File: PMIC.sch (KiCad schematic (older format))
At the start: 63 parts

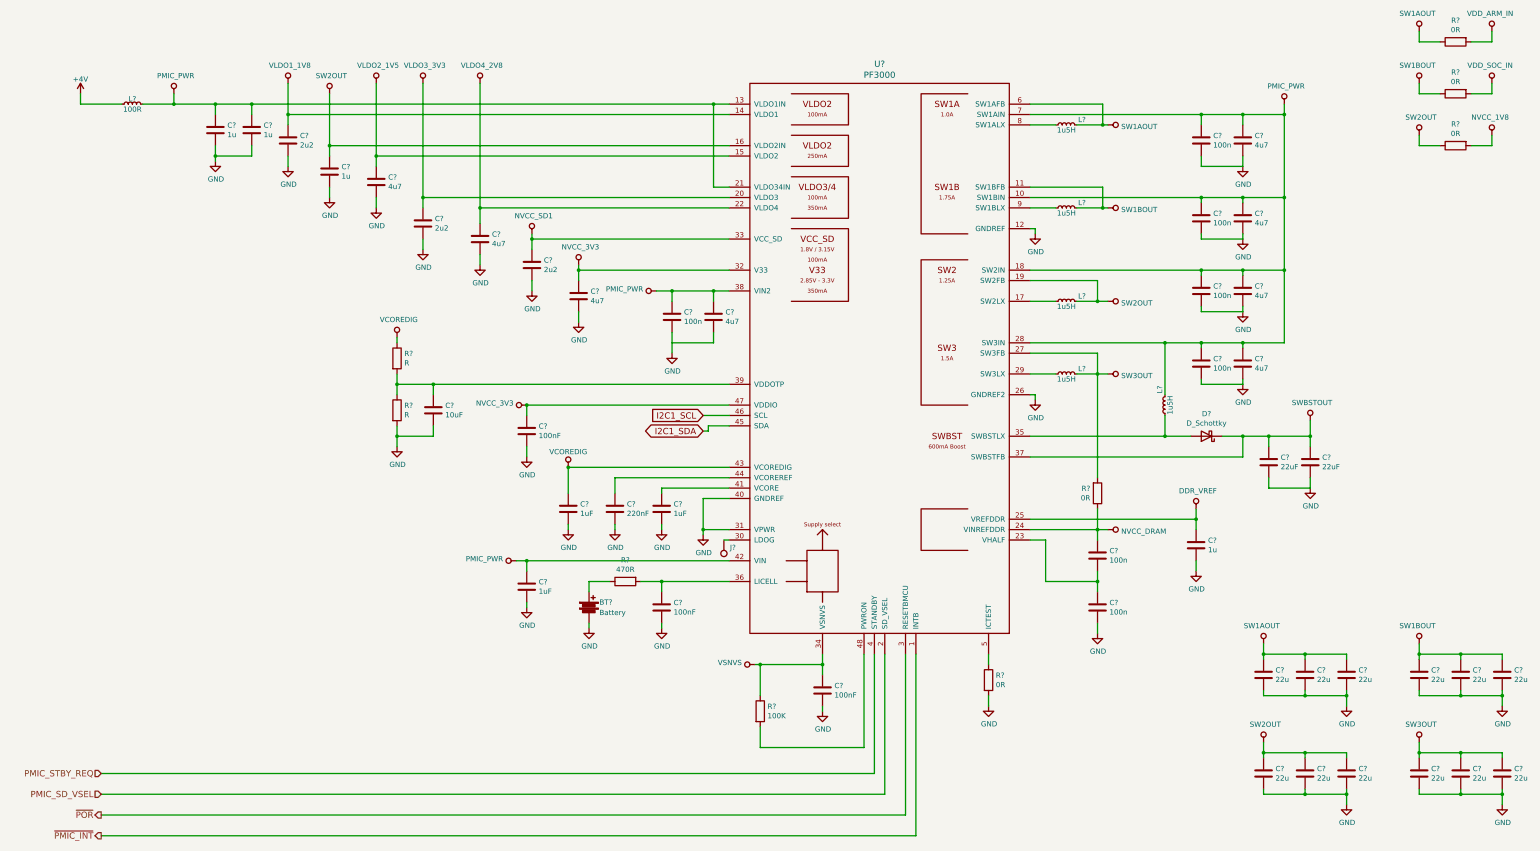
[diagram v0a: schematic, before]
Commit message: modified adui circuit
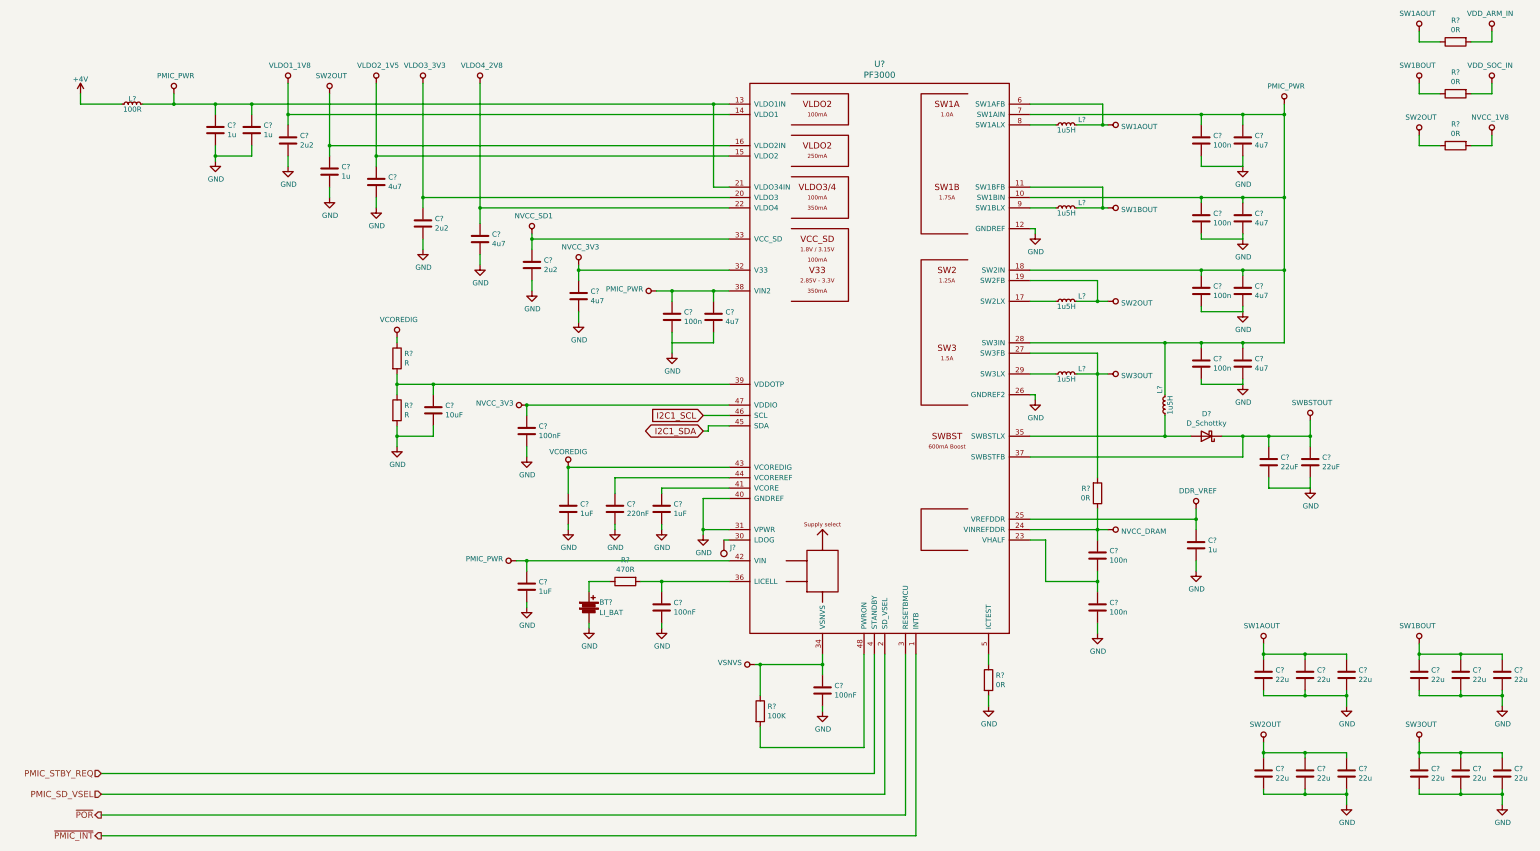
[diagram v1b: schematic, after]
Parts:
- removed BT?: Battery, symbol Battery
- added BT?: LI_BAT, symbol LI_BAT
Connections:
- net GND: now also BT?.2
- net at R?.1: now also BT?.1
